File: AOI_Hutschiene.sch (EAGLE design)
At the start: 33 parts, among them IC1 l4940, SW1 EC12E_SW

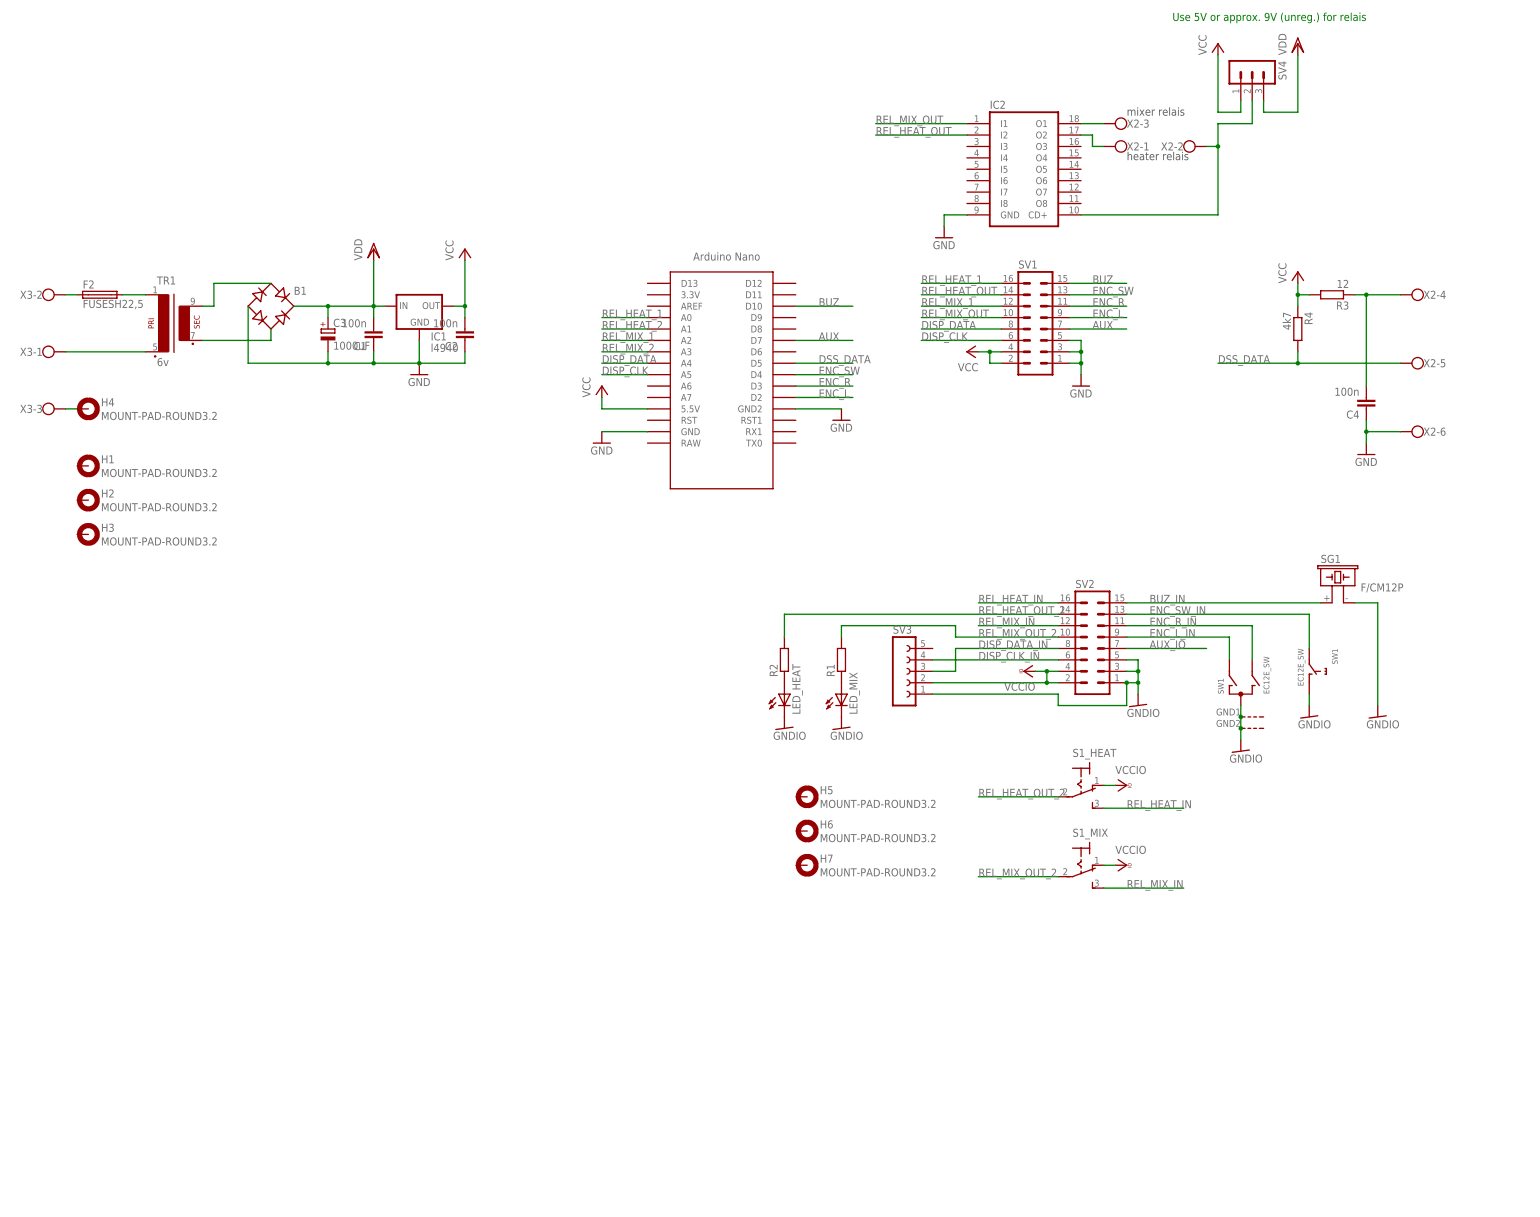
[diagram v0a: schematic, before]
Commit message: updated design
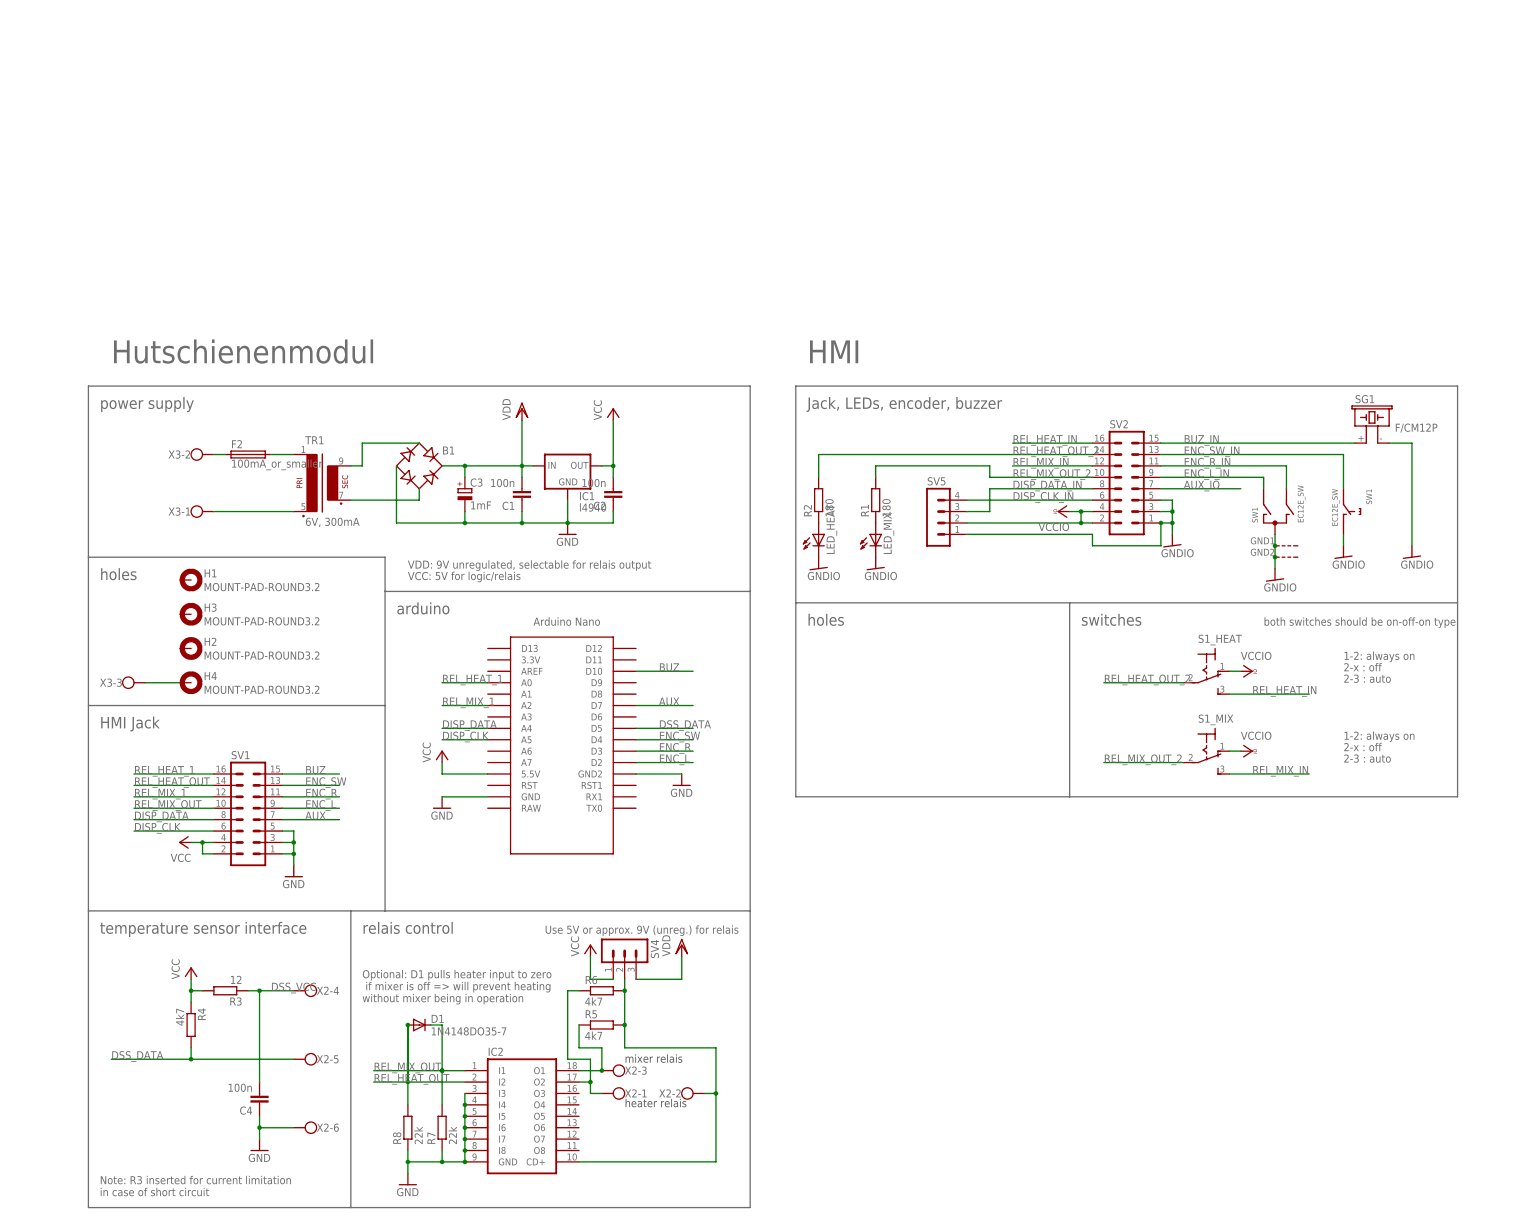
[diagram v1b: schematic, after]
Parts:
- removed H5, H6, H7: MOUNT-PAD-ROUND3.2, holes:MOUNT-PAD-ROUND3.2
- removed SV3: (no value), con-lsta:FE05W
- added D1: 1N4148DO35-7, diode:1N4148DO35-7
- added R5, R6: 4k7, resistor:R-EU_0207/2V
- added R7, R8: 22k, resistor:R-EU_0207/10
- added SV5: (no value), con-lstb:MA04-1
- C3: value 1000uF -> 1mF
- F2: value FUSESH22,5 -> 100mA_or_smaller
- R1, R2: value (none) -> 180
- TR1: value 6v -> 6V, 300mA
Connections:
- net N$12 renamed DSS_VCC
- removed net REL_HEAT_2: U$1.A1
- removed net REL_MIX_2: U$1.A3
- net DISP_CLK_IN: now also SV5.4; no longer SV3.4
- net DISP_DATA_IN: now also SV5.3; no longer SV3.3
- net GND: now also IC2.I3, IC2.I4, IC2.I5, IC2.I6, IC2.I7, IC2.I8, R7.1, R8.1
- net GNDIO: now also SV5.1; no longer SV3.1
- net N$1: now also R5.2, R6.2
- net N$2: now also R5.1
- net N$3: now also R6.1
- net REL_HEAT_OUT: now also D1.A, R8.2
- net REL_MIX_OUT: now also D1.C, R7.2
- net VCCIO: now also SV5.2; no longer SV3.2
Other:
- note added: "1-2: always on"
- note added: "2-3 : auto"
- note added: "2-x : off"
- note added: "HMI"
- note added: "HMI Jack"
- note added: "Hutschienenmodul"
- note added: "Jack, LEDs, encoder, buzzer"
- note added: "Note: R3 inserted for current limitation in case of short circuit"
- note added: "Optional: D1 pulls heater input to zero if mixer is off => will prevent heating without mixer being in operation"
- note added: "VCC: 5V for logic/relais"
- note added: "VDD: 9V unregulated, selectable for relais output"
- note added: "arduino"
- note added: "both switches should be on-off-on type"
- note added: "holes"
- note added: "power supply"
- note added: "relais control"
- note added: "switches"
- note added: "temperature sensor interface"
- moved on the sheet: B1, C1, C2, C3, C4, F2, H1, H2, H3, H4, IC1, IC2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
